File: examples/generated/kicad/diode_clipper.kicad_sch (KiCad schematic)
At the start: 3 parts

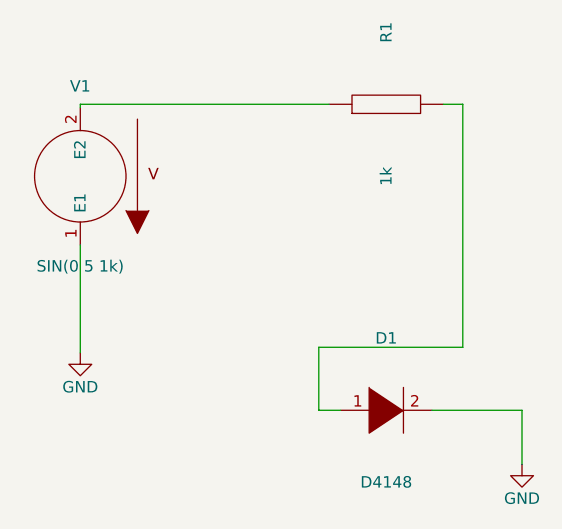
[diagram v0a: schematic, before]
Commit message: Attempt to fix more terminal issues.
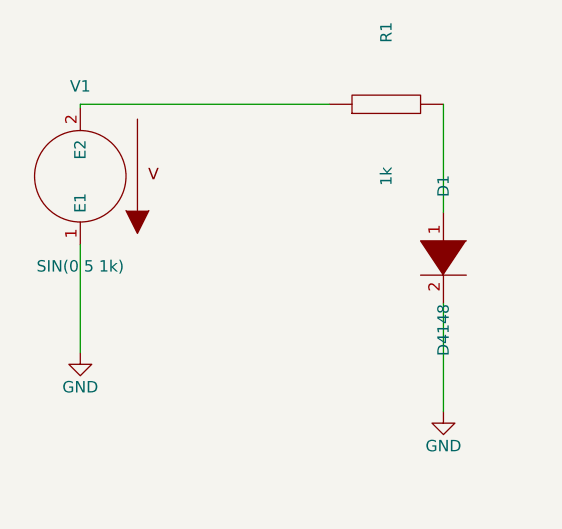
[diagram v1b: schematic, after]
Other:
- moved on the sheet: D1
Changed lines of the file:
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@@
+    )
+  )
+  (symbol (lib_id "GND") (at 56.00 105.62 0) (unit 1)
+    (in_bom yes) (on_board yes)
+    (property "Reference" "#PWR0001" (at 56.0 101.81 0)
+      (effects (font (size 1.27 1.27)) hide)
+    )
+    (property "Value" "GND" (at 56.0 109.43 0)
+      (effects (font (size 1.27 1.27)))
+    )
+    (property "Footprint" "" (at 0 0 0)
+      (effects (font (size 1.27 1.27)) hide)
+    )
+    (property "Datasheet" "" (at 0 0 0)
+      (effects (font (size 1.27 1.27)) hide)
     )
   )
@@
     )
   )
-  (symbol (lib_id "DIODE") (at 90.00 112.00 0) (unit 1)
+  (symbol (lib_id "DIODE") (at 96.35 95.08 270) (unit 1)
     (in_bom yes) (on_board yes)
-    (property "Reference" "D1" (at 90.0 104.0 0)
+    (property "Reference" "D1" (at 96.35 87.08 0)
       (effects (font (size 1.27 1.27)))
     )
-    (property "Value" "D4148" (at 90.0 120.0 0)
+    (property "Value" "D4148" (at 96.35 103.08 0)
       (effects (font (size 1.27 1.27)))
     )
@@
     )
   )
-  (symbol (lib_id "GND") (at 56.00 105.62 0) (unit 1)
+  (symbol (lib_id "GND") (at 96.35 112.16 0) (unit 1)
     (in_bom yes) (on_board yes)
-    (property "Reference" "#PWR0001" (at 56.0 101.81 0)
+    (property "Reference" "#PWR0002" (at 96.35 108.35 0)
       (effects (font (size 1.27 1.27)) hide)
     )
-    (property "Value" "GND" (at 56.0 109.43 0)
+    (property "Value" "GND" (at 96.35 115.97 0)
       (effects (font (size 1.27 1.27)))
     )
@@
     )
   )
-  (symbol (lib_id "GND") (at 105.08 118.00 0) (unit 1)
-    (in_bom yes) (on_board yes)
-    (property "Reference" "#PWR0002" (at 105.08 114.19 0)
-      (effects (font (size 1.27 1.27)) hide)
-    )
-    (property "Value" "GND" (at 105.08 121.81 0)
-      (effects (font (size 1.27 1.27)))
-    )
-    (property "Footprint" "" (at 0 0 0)
-      (effects (font (size 1.27 1.27)) hide)
-    )
-    (property "Datasheet" "" (at 0 0 0)
-      (effects (font (size 1.27 1.27)) hide)
-    )
+  (wire (pts (xy 96.35 100.16) (xy 96.35 112.16))
+    (stroke (width 0) (type solid) (color 0 0 0 0))
   )
   (wire (pts (xy 56.00 93.62) (xy 56.00 105.62))
-    (stroke (width 0) (type solid) (color 0 0 0 0))
-  )
-  (wire (pts (xy 95.08 112.00) (xy 105.08 112.00))
-    (stroke (width 0) (type solid) (color 0 0 0 0))
-  )
-  (wire (pts (xy 105.08 112.00) (xy 105.08 118.00))
     (stroke (width 0) (type solid) (color 0 0 0 0))
   )
@@
     (stroke (width 0) (type solid) (color 0 0 0 0))
   )
-  (wire (pts (xy 96.35 78.00) (xy 98.50 78.00))
-    (stroke (width 0) (type solid) (color 0 0 0 0))
-  )
-  (wire (pts (xy 98.50 78.00) (xy 98.50 105.00))
-    (stroke (width 0) (type solid) (color 0 0 0 0))
-  )
-  (wire (pts (xy 98.50 105.00) (xy 82.50 105.00))
-    (stroke (width 0) (type solid) (color 0 0 0 0))
-  )
-  (wire (pts (xy 82.50 105.00) (xy 82.50 112.00))
-    (stroke (width 0) (type solid) (color 0 0 0 0))
-  )
-  (wire (pts (xy 82.50 112.00) (xy 84.92 112.00))
+  (wire (pts (xy 96.35 78.00) (xy 96.35 90.00))
     (stroke (width 0) (type solid) (color 0 0 0 0))
   )
@@
   (symbol_instances
     (path "/2c9e1e1c-69f0-5312-966c-7e56fb048925" (reference "V1") (unit 1) (value "SIN(0 5 1k)") (footprint ""))
+    (path "/229331e1-49b2-5d63-84c6-e3f127e9d83d" (reference "#PWR0001") (unit 1) (value "GND") (footprint ""))
     (path "/2c8aff2b-0935-51d8-b11f-1b19ccafeed0" (reference "R1") (unit 1) (value "1k") (footprint ""))
     (path "/6d337348-46f7-501d-8787-9fc457eabff9" (reference "D1") (unit 1) (value "D4148") (footprint ""))
-    (path "/229331e1-49b2-5d63-84c6-e3f127e9d83d" (reference "#PWR0001") (unit 1) (value "GND") (footprint ""))
     (path "/331ec4ee-80da-5867-9867-b03498e7d5de" (reference "#PWR0002") (unit 1) (value "GND") (footprint ""))
   )
